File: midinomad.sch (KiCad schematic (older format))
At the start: 47 parts, among them U1 6N138

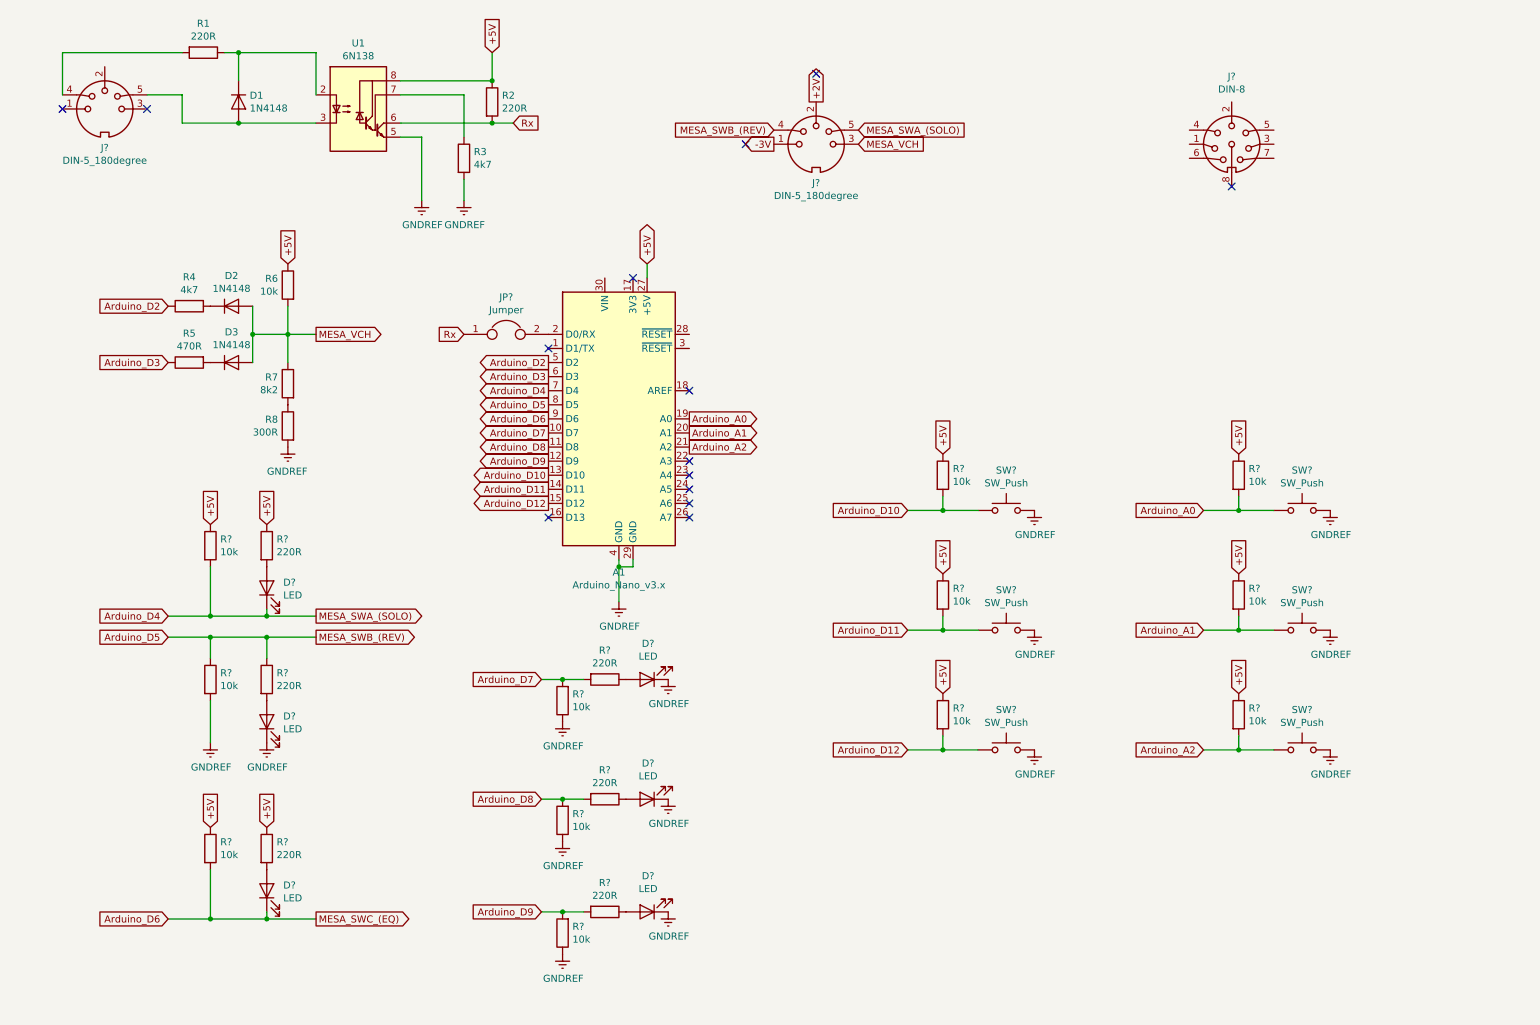
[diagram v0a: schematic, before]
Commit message: Updated schematics. Still work in progress.
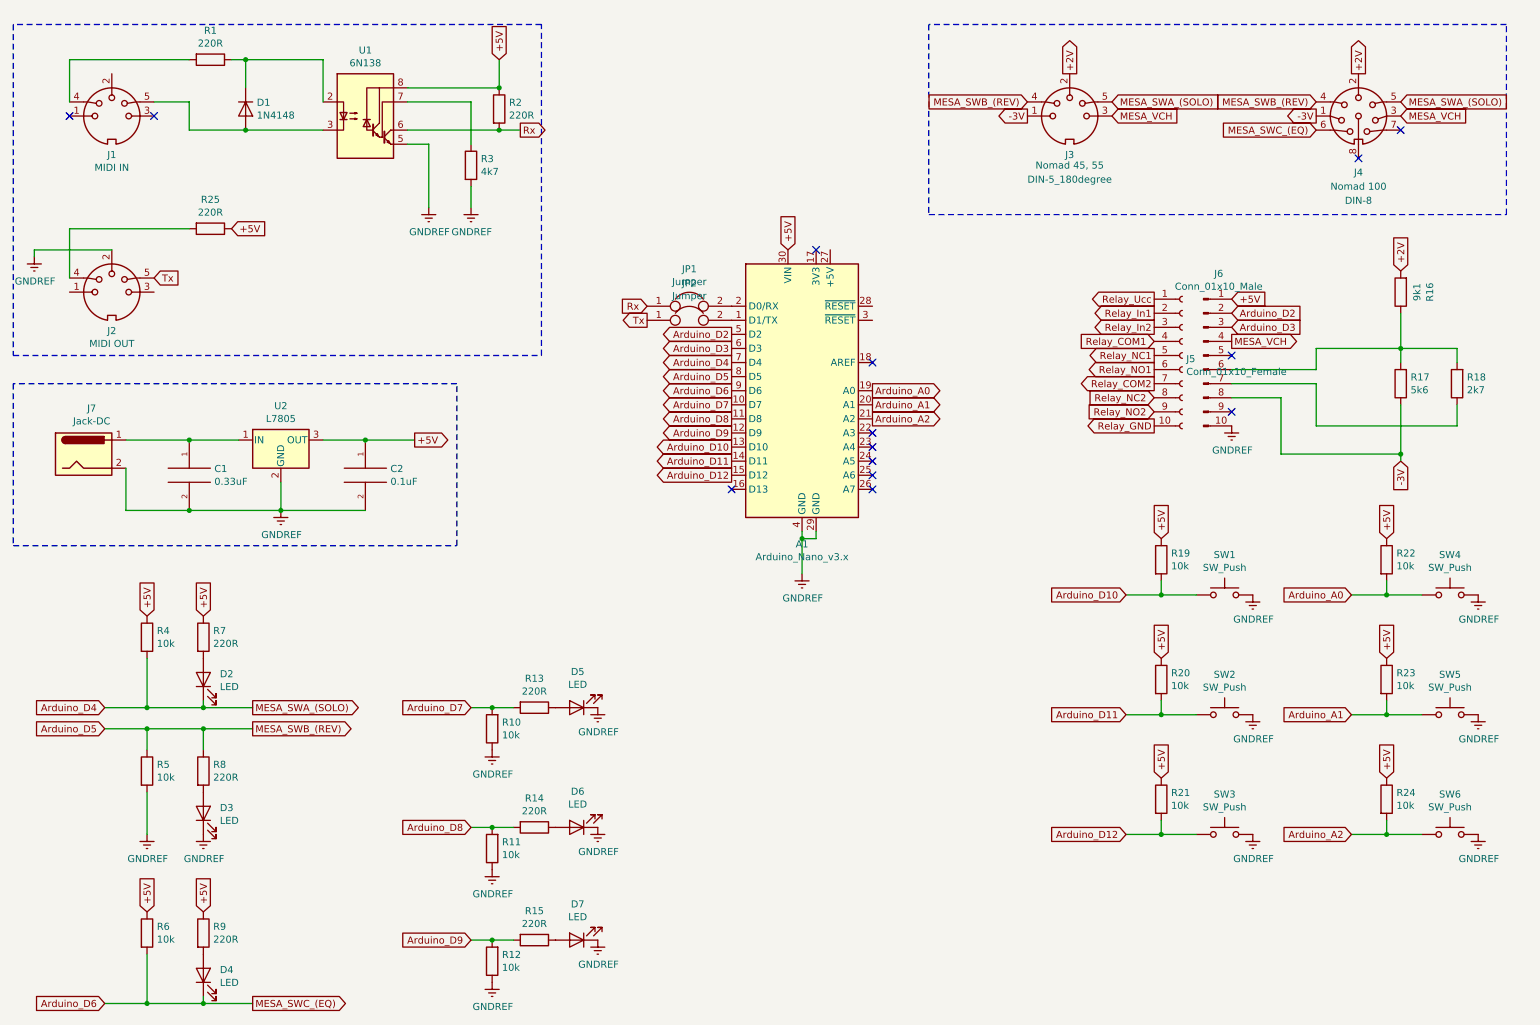
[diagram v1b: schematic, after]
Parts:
- removed D2, D3: 1N4148, Diode_THT:D_DO-35_SOD27_P7.62mm_Horizontal, symbol Diode:1N4148
- removed R4: 4k7, symbol Device:R
- removed R5: 470R, symbol Device:R
- removed R6: 10k, symbol Device:R
- removed R7: 8k2, symbol Device:R
- removed R8: 300R, symbol Device:R
- added C1: 0.33uF, symbol pspice:C
- added C2: 0.1uF, symbol pspice:C
- added J2: MIDI OUT, w_conn_av:din-5, symbol Connector:DIN-5_180degree
- added J5: Conn_01x10_Female, symbol Connector:Conn_01x10_Female
- added J6: Conn_01x10_Male, symbol Connector:Conn_01x10_Male
- added J7: Jack-DC, symbol Connector:Jack-DC
- added JP2: Jumper, Connector_PinHeader_2.54mm:PinHeader_1x02_P2.54mm_Vertical, symbol Device:Jumper
- added R16: 9k1, Resistor_THT:R_Axial_DIN0207_L6.3mm_D2.5mm_P10.16mm_Horizontal, symbol Device:R
- added R17: 5k6, Resistor_THT:R_Axial_DIN0207_L6.3mm_D2.5mm_P10.16mm_Horizontal, symbol Device:R
- added R18: 2k7, Resistor_THT:R_Axial_DIN0207_L6.3mm_D2.5mm_P10.16mm_Horizontal, symbol Device:R
- added R25: 220R, Resistor_THT:R_Axial_DIN0207_L6.3mm_D2.5mm_P10.16mm_Horizontal, symbol Device:R
- added U2: L7805, symbol Regulator_Linear:L7805
- D2, D3, D4, D5, D6, D7: renamed from D?; footprint (none) -> LED_THT:LED_D5.0mm
- J1: renamed from J?; value DIN-5_180degree -> MIDI IN; footprint (none) -> w_conn_av:din-5
- J3: renamed from J?; footprint (none) -> w_conn_av:din-5; Note (none) -> Nomad 45, 55
- J4: renamed from J?; footprint (none) -> Connector_PinHeader_2.54mm:PinHeader_1x07_P2.54mm_Vertical; Note (none) -> Nomad 100
- JP1: renamed from JP?; footprint (none) -> Connector_PinHeader_2.54mm:PinHeader_1x02_P2.54mm_Vertical
- R1, R2, R3: footprint (none) -> Resistor_THT:R_Axial_DIN0207_L6.3mm_D2.5mm_P10.16mm_Horizontal
- R10, R11, R12, R13, R14, R15, R19, R20, R21, R22, R23, R24, R4, R5, R6, R7, R8, R9: renamed from R?; footprint (none) -> Resistor_THT:R_Axial_DIN0207_L6.3mm_D2.5mm_P10.16mm_Horizontal
- SW1, SW2, SW3, SW4, SW5, SW6: renamed from SW?; footprint (none) -> Button_Switch_THT:SW_PUSH_6mm
- U1: footprint (none) -> Package_DIP:DIP-8_W7.62mm
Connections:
- net +2V: now also J4.2, R16.2
- net +5V: now also A1.30 (VIN), C2.1, J6.1 (Pin_1), R25.1, U2.3 (OUT); no longer A1.27 (+5V)
- net -3V: now also J4.1, J6.8 (Pin_8), R17.1
- net Arduino_D2: now also J6.2 (Pin_2)
- net Arduino_D3: now also J6.3 (Pin_3)
- net Arduino_D4: now also J4.5
- net Arduino_D5: now also J4.4
- net Arduino_D6: now also J4.6
- net GNDREF: now also C1.2, C2.2, J2.2, J6.10 (Pin_10), J7.2, U2.2 (GND)
- net MESA_VCH: now also J4.3, J6.4 (Pin_4)
- net at A1.1 (D1/TX): now also JP2.2
- new net: J6.6 (Pin_6), R16.1, R17.2, R18.2
- new net: J6.7 (Pin_7), R18.1
- new net: C1.1, J7.1, U2.1 (IN)
- new net: J2.4, R25.2
- new net Relay_COM1: J5.4 (Pin_4)
- new net Relay_COM2: J5.7 (Pin_7)
- new net Relay_GND: J5.10 (Pin_10)
- new net Relay_In1: J5.2 (Pin_2)
- new net Relay_In2: J5.3 (Pin_3)
- new net Relay_NC1: J5.5 (Pin_5)
- new net Relay_NC2: J5.8 (Pin_8)
- new net Relay_NO1: J5.6 (Pin_6)
- new net Relay_NO2: J5.9 (Pin_9)
- new net Relay_Ucc: J5.1 (Pin_1)
- new net Tx: J2.5, JP2.1
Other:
- moved on the sheet: A1, D1, D2, D3, D4, D5, D6, D7, J1, J3, J4, JP1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
